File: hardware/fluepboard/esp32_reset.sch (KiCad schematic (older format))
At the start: 2 parts, among them U4 UMH3N

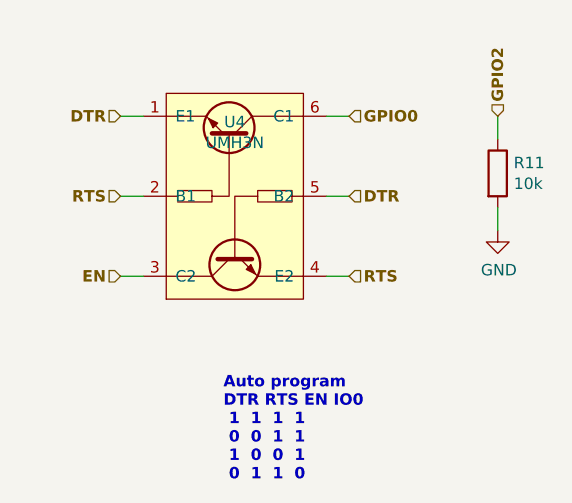
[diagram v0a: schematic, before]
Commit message: Commit jlcpcb compatible version
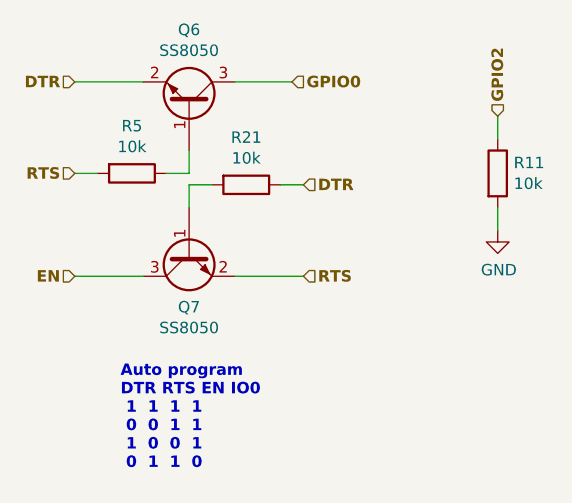
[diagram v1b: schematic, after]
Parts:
- removed U4: UMH3N, Package_TO_SOT_SMD:SOT-363_SC-70-6, symbol fluepdot:UMH3N
- added Q6, Q7: SS8050, Package_TO_SOT_SMD:SOT-23, symbol Device:Q_NPN_BEC
- added R21, R5: 10k, Resistor_SMD:R_0603_1608Metric, symbol Device:R
- R11: footprint Resistor_SMD:R_0805_2012Metric -> Resistor_SMD:R_0603_1608Metric; Description (none) -> CHIP RESISTOR - SURFACE MOUNT 10KOHMS ±1% 1/10W 0603 ROHS; Extended Part (none) -> 0; LCSC (none) -> C25804; Manufacturer (none) -> 0603WAF1002T5E
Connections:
- net DTR: now also Q6.2 (E), R21.1
- net EN: now also Q7.3 (C)
- net GPIO0: now also Q6.3 (C)
- net RTS: now also Q7.2 (E), R5.2
- new net: Q6.1 (B), R5.1
- new net: Q7.1 (B), R21.2
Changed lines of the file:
@@
 EESchema Schematic File Version 4
 LIBS:fluepdot-cache
-EELAYER 29 0
+EELAYER 30 0
 EELAYER END
 $Descr A4 11693 8268
@@
 Comment4 ""
 $EndDescr
-Text HLabel 1350 1350 0    50   Input ~ 10
-RTS
-Text HLabel 1350 1000 0    50   Input ~ 10
-DTR
-Text HLabel 2350 1000 2    50   Input ~ 10
-GPIO0
-$Comp
-L fluepdot:UMH3N U4
-U 1 1 5CAE7BF5
-P 1850 1350
-F 0 "U4" H 1850 1675 50  0000 C CNN
-F 1 "UMH3N" H 1850 1584 50  0000 C CNN
-F 2 "Package_TO_SOT_SMD:SOT-363_SC-70-6" H 1850 1350 50  0001 C CNN
-F 3 "" H 1850 1350 50  0001 C CNN
-F 4 "UMH3NTN" H 1850 1350 50  0001 C CNN "Octopart"
-	1    1850 1350
-	1    0    0    -1
-$EndComp
-Text HLabel 2350 1700 2    50   Input ~ 10
-RTS
-Wire Wire Line
-	1350 1350 1450 1350
-Wire Wire Line
-	2250 1700 2350 1700
-Wire Wire Line
-	1350 1000 1450 1000
-Text HLabel 2350 1350 2    50   Input ~ 10
-DTR
-Wire Wire Line
-	2350 1350 2250 1350
-Wire Wire Line
-	2350 1000 2250 1000
-Text HLabel 1350 1700 0    50   Input ~ 10
-EN
-Wire Wire Line
-	1350 1700 1450 1700
-Text Notes 1800 2600 0    50   ~ 10
+Text Notes 1350 2550 0    50   ~ 10
 Auto program\nDTR RTS EN IO0\n 1  1  1  1\n 0  0  1  1\n 1  0  0  1\n 0  1  1  0\n
 $Comp
@@
 F 0 "R11" H 3070 1296 50  0000 L CNN
 F 1 "10k" H 3070 1205 50  0000 L CNN
-F 2 "Resistor_SMD:R_0805_2012Metric" V 2930 1250 50  0001 C CNN
+F 2 "Resistor_SMD:R_0603_1608Metric" V 2930 1250 50  0001 C CNN
 F 3 "~" H 3000 1250 50  0001 C CNN
 F 4 "RC0805FR-0710KL" H 3000 1250 50  0001 C CNN "Octopart"
+F 5 "C25804" H 3000 1250 50  0001 C CNN "LCSC"
+F 6 "0603WAF1002T5E" H 3000 1250 50  0001 C CNN "Manufacturer"
+F 7 "0" H 3000 1250 50  0001 C CNN "Extended Part"
+F 8 "CHIP RESISTOR - SURFACE MOUNT 10KOHMS ±1% 1/10W 0603 ROHS" H 3000 1250 50  0001 C CNN "Description"
 	1    3000 1250
 	1    0    0    -1
@@
 Wire Wire Line
 	3000 1500 3000 1400
+Text HLabel 1150 850  0    50   Input ~ 10
+DTR
+Text HLabel 1150 1250 0    50   Input ~ 10
+RTS
+$Comp
+L Device:R R5
+U 1 1 5D99E9E6
+P 1400 1250
+F 0 "R5" V 1193 1250 50  0000 C CNN
+F 1 "10k" V 1284 1250 50  0000 C CNN
+F 2 "Resistor_SMD:R_0603_1608Metric" V 1330 1250 50  0001 C CNN
+F 3 "~" H 1400 1250 50  0001 C CNN
+F 4 "CHIP RESISTOR - SURFACE MOUNT 10KOHMS ±1% 1/10W 0603 ROHS" H 1400 1250 50  0001 C CNN "Description"
+F 5 "0" H 1400 1250 50  0001 C CNN "Extended Part"
+F 6 "C25804" H 1400 1250 50  0001 C CNN "LCSC"
+F 7 "0603WAF1002T5E" H 1400 1250 50  0001 C CNN "Manufacturer"
+	1    1400 1250
+	0    1    1    0
+$EndComp
+Wire Wire Line
+	1150 850  1450 850
+Wire Wire Line
+	1150 1250 1250 1250
+Wire Wire Line
+	1550 1250 1650 1250
+Wire Wire Line
+	1650 1250 1650 1150
+Text HLabel 2100 850  2    50   Input ~ 10
+GPIO0
+Wire Wire Line
+	1850 850  2100 850
+$Comp
+L Device:R R21
+U 1 1 5D9A1B1E
+P 1900 1300
+F 0 "R21" V 1693 1300 50  0000 C CNN
+F 1 "10k" V 1784 1300 50  0000 C CNN
+F 2 "Resistor_SMD:R_0603_1608Metric" V 1830 1300 50  0001 C CNN
+F 3 "~" H 1900 1300 50  0001 C CNN
+F 4 "CHIP RESISTOR - SURFACE MOUNT 10KOHMS ±1% 1/10W 0603 ROHS" H 1900 1300 50  0001 C CNN "Description"
+F 5 "0" H 1900 1300 50  0001 C CNN "Extended Part"
+F 6 "C25804" H 1900 1300 50  0001 C CNN "LCSC"
+F 7 "0603WAF1002T5E" H 1900 1300 50  0001 C CNN "Manufacturer"
+	1    1900 1300
+	0    1    1    0
+$EndComp
+Wire Wire Line
+	1650 1400 1650 1300
+Wire Wire Line
+	1650 1300 1750 1300
+Text HLabel 2150 1300 2    50   Input ~ 10
+DTR
+Wire Wire Line
+	2050 1300 2150 1300
+Text HLabel 2150 1700 2    50   Input ~ 10
+RTS
+Wire Wire Line
+	1850 1700 2150 1700
+Text HLabel 1150 1700 0    50   Input ~ 10
+EN
+Wire Wire Line
+	1150 1700 1450 1700
+$Comp
+L Device:Q_NPN_BEC Q6
+U 1 1 5D9AA5F7
+P 1650 950
+F 0 "Q6" V 1978 950 50  0000 C CNN
+F 1 "SS8050" V 1887 950 50  0000 C CNN
+F 2 "Package_TO_SOT_SMD:SOT-23" H 1850 1050 50  0001 C CNN
+F 3 "~" H 1650 950 50  0001 C CNN
+F 4 "TRANSISTORS (NPN/PNP) NPN 1.5A 25V SOT-23(SOT-23-3) ROHS" H 1650 950 50  0001 C CNN "Description"
+F 5 "0" H 1650 950 50  0001 C CNN "Extended Part"
+F 6 "C2150" H 1650 950 50  0001 C CNN "LCSC"
+	1    1650 950
+	0    1    -1   0
+$EndComp
+$Comp
+L Device:Q_NPN_BEC Q7
+U 1 1 5D9ADB8D
+P 1650 1600
+F 0 "Q7" V 1885 1600 50  0000 C CNN
+F 1 "SS8050" V 1976 1600 50  0000 C CNN
+F 2 "Package_TO_SOT_SMD:SOT-23" H 1850 1700 50  0001 C CNN
+F 3 "~" H 1650 1600 50  0001 C CNN
+F 4 "TRANSISTORS (NPN/PNP) NPN 1.5A 25V SOT-23(SOT-23-3) ROHS" H 1650 1600 50  0001 C CNN "Description"
+F 5 "0" H 1650 1600 50  0001 C CNN "Extended Part"
+F 6 "C2150" H 1650 1600 50  0001 C CNN "LCSC"
+	1    1650 1600
+	0    -1   1    0
+$EndComp
 $EndSCHEMATC
